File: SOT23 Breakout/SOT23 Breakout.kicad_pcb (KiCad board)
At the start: 2 copper layers, 17.5 x 10 mm, 8 parts, among them J1 IO, J2 IO, J3 ANC, J4 ANC, Q1 NMOS, Q2 NMOS, Q3 NMOS, Q4 NMOS

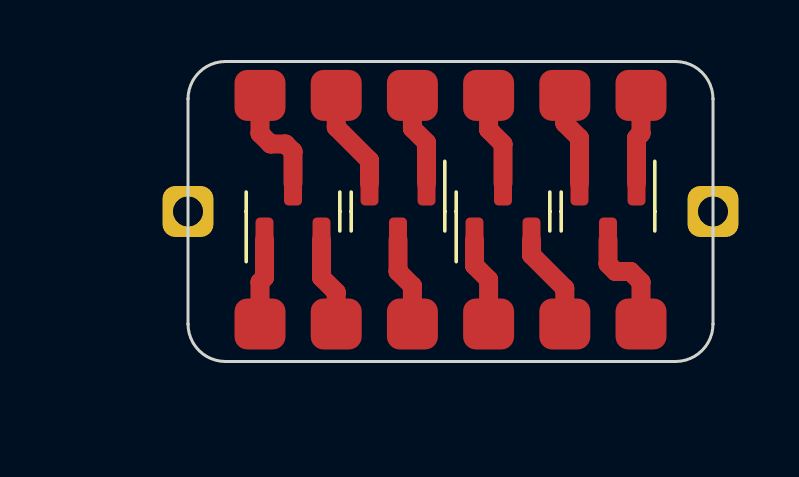
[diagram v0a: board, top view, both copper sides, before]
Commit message: Updated Files
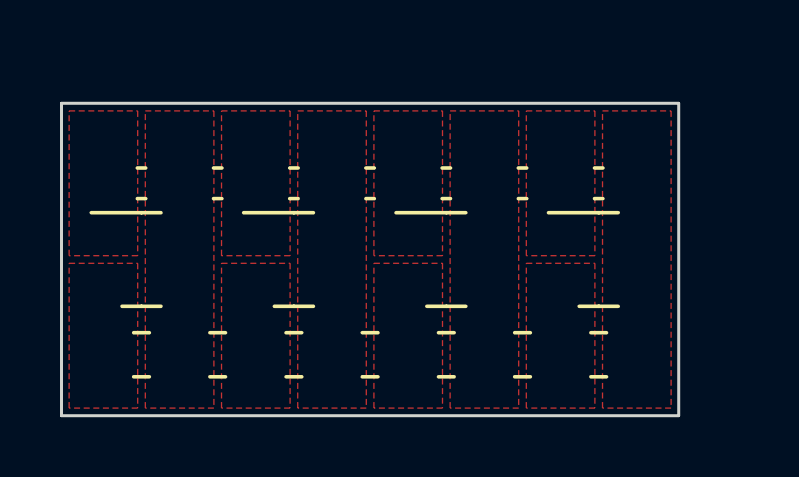
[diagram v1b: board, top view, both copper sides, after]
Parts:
- removed J1, J2: IO, Connector_PinHeader_2.54mm:PinHeader_1x06_P2.54mm_Vertical
- removed J3, J4: ANC, Connector_PinHeader_2.54mm:PinHeader_1x01_P2.54mm_Vertical
- removed Q1, Q2, Q3, Q4: NMOS, Package_TO_SOT_SMD:SOT-23
- added REF**: C_0603_1608Metric, Capacitor_SMD:C_0603_1608Metric, F.Cu at (139.7, 99.1)
- added REF**: C_0603_1608Metric, Capacitor_SMD:C_0603_1608Metric, F.Cu at (144.8, 99.1)
- added REF**: SOT-23, Package_TO_SOT_SMD:SOT-23, F.Cu at (139.7, 101.6)
- added REF**: SOT-23, Package_TO_SOT_SMD:SOT-23, F.Cu at (144.8, 101.6)
- added REF**: C_0603_1608Metric, Capacitor_SMD:C_0603_1608Metric, F.Cu at (142.2, 99.1)
- added REF**: C_0805_2012Metric, Capacitor_SMD:C_0805_2012Metric, F.Cu at (144.8, 104.8)
- added REF**: C_0805_2012Metric, Capacitor_SMD:C_0805_2012Metric, F.Cu at (147.3, 104.8)
- added REF**: C_0805_2012Metric, Capacitor_SMD:C_0805_2012Metric, F.Cu at (139.7, 104.8)
- added REF**: C_0603_1608Metric, Capacitor_SMD:C_0603_1608Metric, F.Cu at (147.3, 99.1)
- added REF**: SOT-23, Package_TO_SOT_SMD:SOT-23, F.Cu at (154.9, 101.6)
- added REF**: SOT-23, Package_TO_SOT_SMD:SOT-23, F.Cu at (149.9, 101.6)
- added REF**: C_0805_2012Metric, Capacitor_SMD:C_0805_2012Metric, F.Cu at (154.9, 104.8)
- added REF**: C_0805_2012Metric, Capacitor_SMD:C_0805_2012Metric, F.Cu at (142.2, 104.8)
- added REF**: C_0805_2012Metric, Capacitor_SMD:C_0805_2012Metric, F.Cu at (152.4, 104.8)
- added REF**: C_0603_1608Metric, Capacitor_SMD:C_0603_1608Metric, F.Cu at (152.4, 99.1)
- added REF**: C_0603_1608Metric, Capacitor_SMD:C_0603_1608Metric, F.Cu at (154.9, 99.1)
- added REF**: C_0603_1608Metric, Capacitor_SMD:C_0603_1608Metric, F.Cu at (149.9, 99.1)
- added REF**: C_0805_2012Metric, Capacitor_SMD:C_0805_2012Metric, F.Cu at (149.9, 104.8)
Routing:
- net Net-(Q1-Pad3): track 3.68 -> 0.00 mm
- net Net-(Q4-Pad3): track 3.56 -> 0.00 mm
- net Net-(J2-Pad2): track 3.39 -> 0.00 mm
- net Net-(Q3-Pad2): track 3.27 -> 0.00 mm
- net Net-(J2-Pad5): track 3.14 -> 0.00 mm
- net Net-(Q3-Pad3): track 3.13 -> 0.00 mm
- net Net-(J2-Pad3): track 3.13 -> 0.00 mm
- net Net-(Q1-Pad2): track 3.02 -> 0.00 mm
- net Net-(Q2-Pad3): track 3.01 -> 0.00 mm
- net Net-(Q3-Pad1): track 3.01 -> 0.00 mm
- net Net-(J2-Pad6): track 2.99 -> 0.00 mm
- net Net-(Q1-Pad1): track 2.87 -> 0.00 mm
- added copper zone on F.Cu, net (none)
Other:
- board size 17.5 x 10 mm -> 20.6 x 10.4 mm
